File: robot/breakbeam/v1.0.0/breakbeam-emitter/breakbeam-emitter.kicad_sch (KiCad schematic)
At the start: 8 parts, among them J1 Conn_01x03, Q1 RUC002N05T116

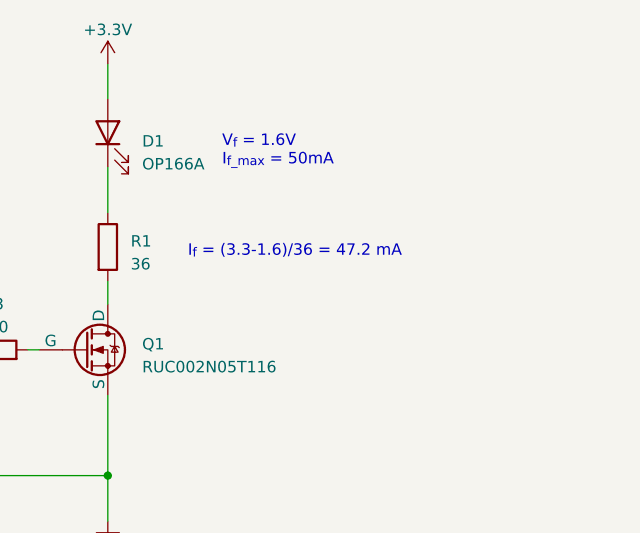
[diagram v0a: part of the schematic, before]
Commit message: Ordering changes
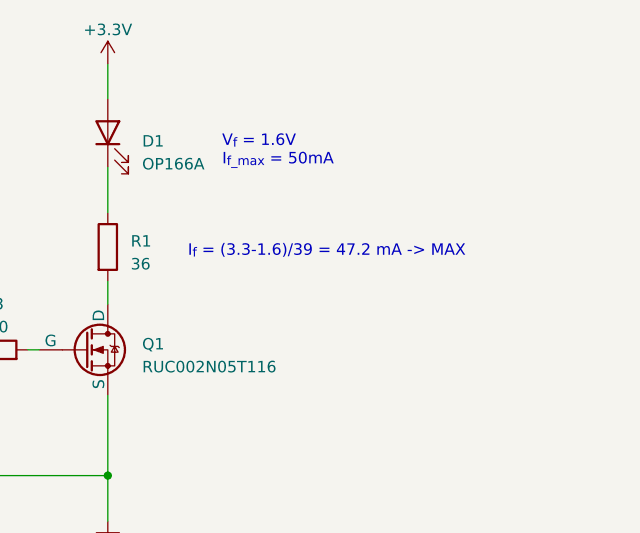
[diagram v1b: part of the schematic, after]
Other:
- note added: "I_{f} = (3.3-1.6)/39 = 47.2 mA -> MAX"
- note removed: "I_{f} = (3.3-1.6)/36 = 47.2 mA"
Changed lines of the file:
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@@
     (stroke (width 0) (type default))
   )
-  (text "I_{f} = (3.3-1.6)/36 = 47.2 mA" (at 193.04 95.25 0)
+  (text "I_{f} = (3.3-1.6)/39 = 47.2 mA -> MAX" (at 193.04 95.25 0)
     (effects (font (size 1.27 1.27)) (justify left bottom))
   )
